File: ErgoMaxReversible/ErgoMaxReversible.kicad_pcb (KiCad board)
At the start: 2 copper layers, 182.8 x 169.2 mm, 106 parts, among them J1 PJ-320A, K1 KEYSW, K10 KEYSW, K11 KEYSW, K12 KEYSW, K13 KEYSW, K14 KEYSW, K15 KEYSW, K16 KEYSW, K17 KEYSW, K18 KEYSW, K19 KEYSW, K2 KEYSW, K20 KEYSW, K21 KEYSW, K22 KEYSW, K23 KEYSW, K24 KEYSW, K25 KEYSW, K26 KEYSW, K27 KEYSW, K28 KEYSW, K29 KEYSW, K3 KEYSW, K30 KEYSW, K31 KEYSW, K32 KEYSW, K33 KEYSW, K34 KEYSW, K35 KEYSW, K36 KEYSW, K37 KEYSW, K38 KEYSW, K39 KEYSW, K4 KEYSW, K40 KEYSW, K41 KEYSW, K42 KEYSW, K43 KEYSW, K44 KEYSW, K5 KEYSW, K6 KEYSW, K7 KEYSW, K8 KEYSW, K9 KEYSW, U1 ProMicro

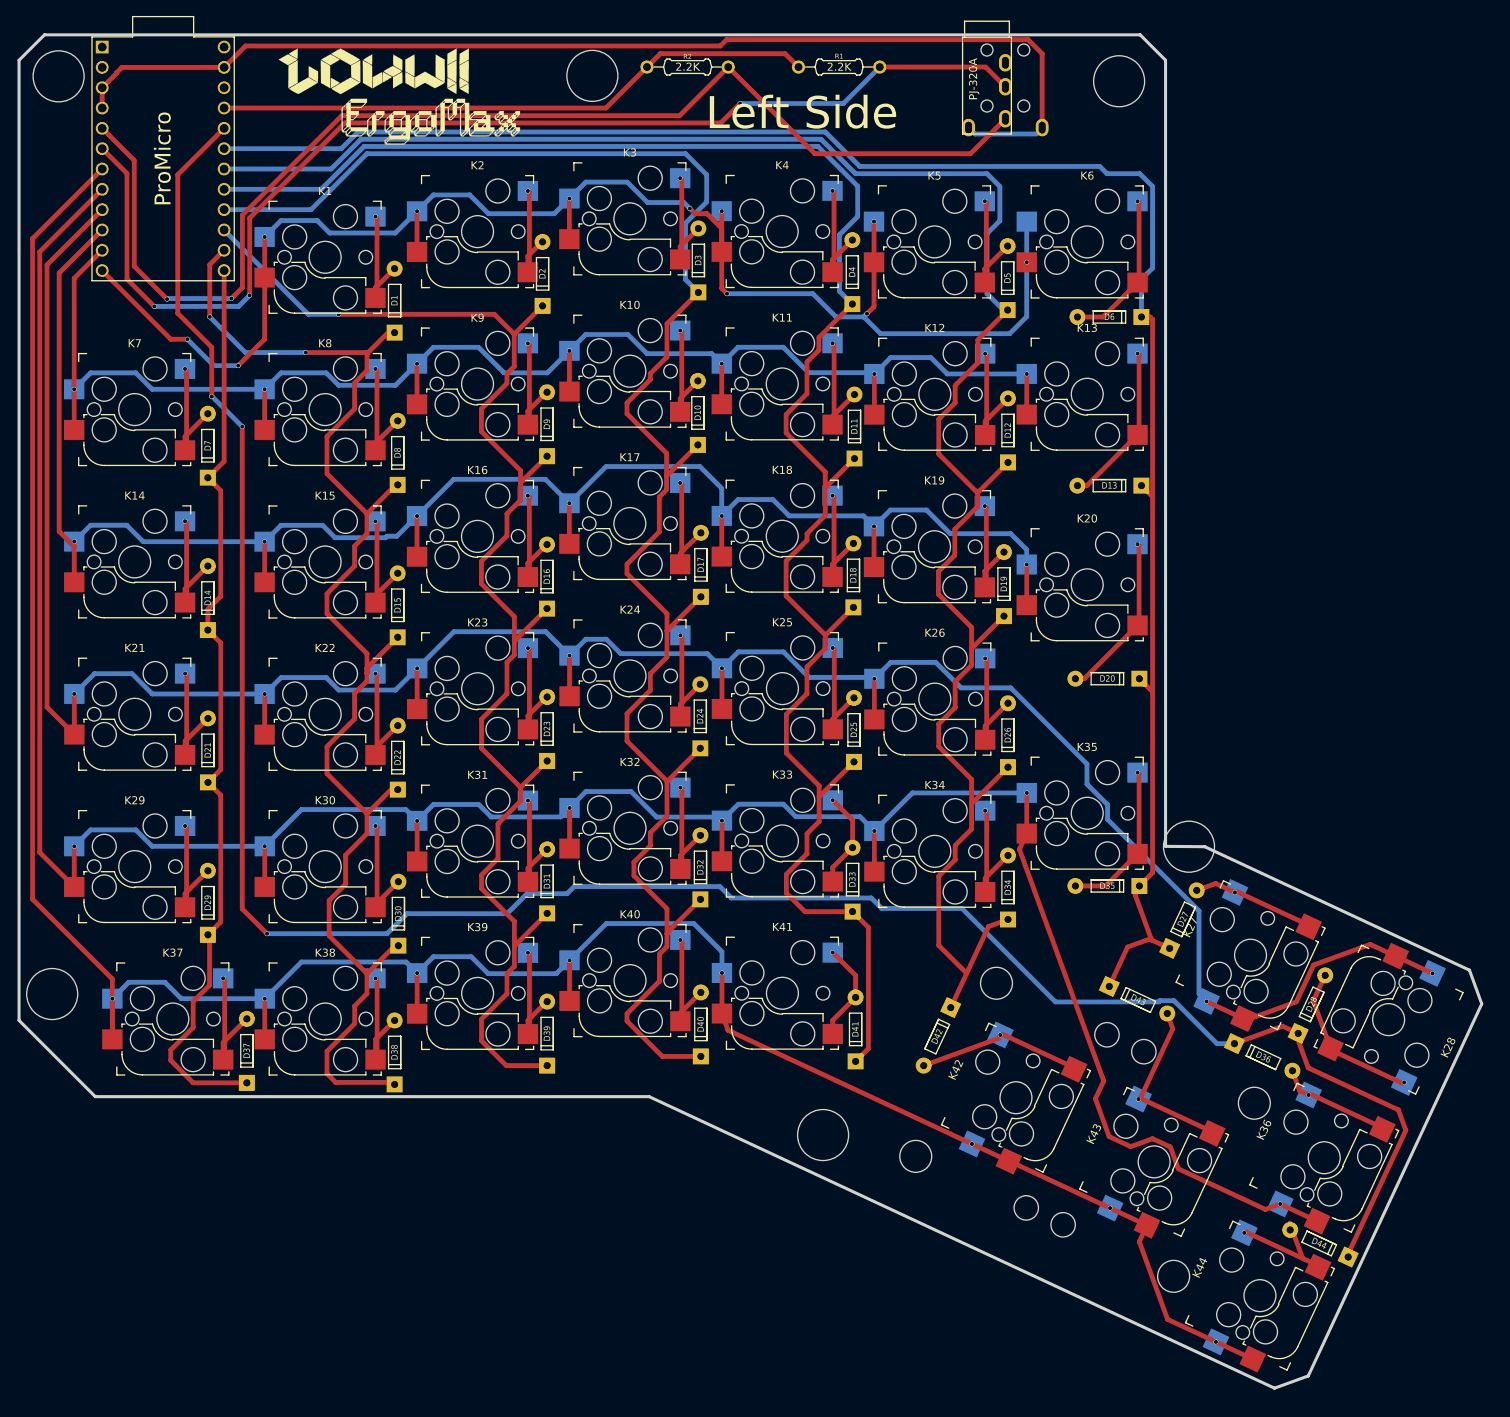
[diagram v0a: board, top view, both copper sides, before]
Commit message: Fix net
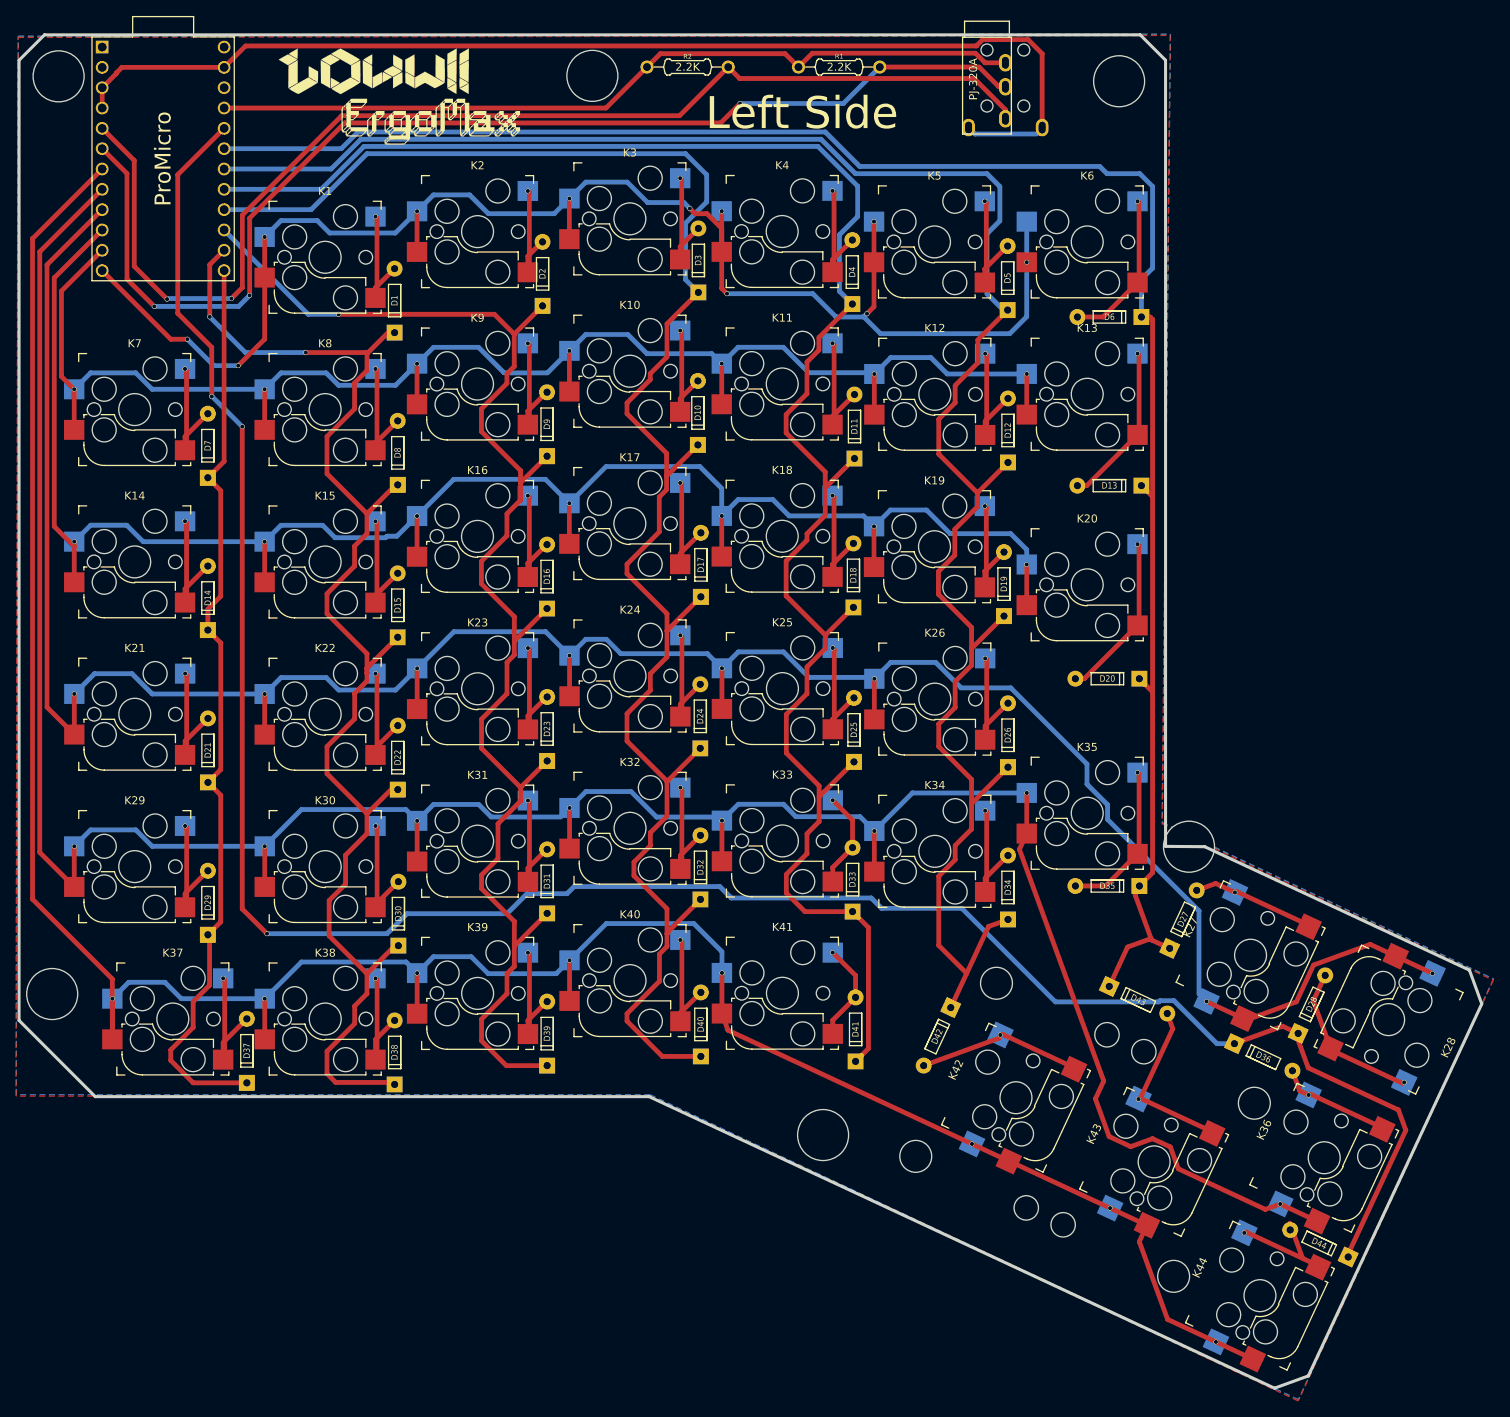
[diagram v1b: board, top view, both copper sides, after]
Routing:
- net VCC: track 75.3 -> 102.4 mm
- net SDA: track 153.1 -> 150.2 mm
- net /Row1: track 187.4 -> 188.7 mm
- net /Row2: track 218.1 -> 218.6 mm
- added copper zone on B.Cu, net GND
- added copper zone on F.Cu, net GND
